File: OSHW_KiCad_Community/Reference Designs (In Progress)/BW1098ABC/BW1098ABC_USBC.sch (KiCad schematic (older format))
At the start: 36 parts, among them J10 USB3.1 TYPEC XKB-U262, J12 PJ-050AH or NEB21R, J13 DF23C-50DP-0.5V_92_, U6 USB Type-C Switch, U7 USB Type-C Port Control

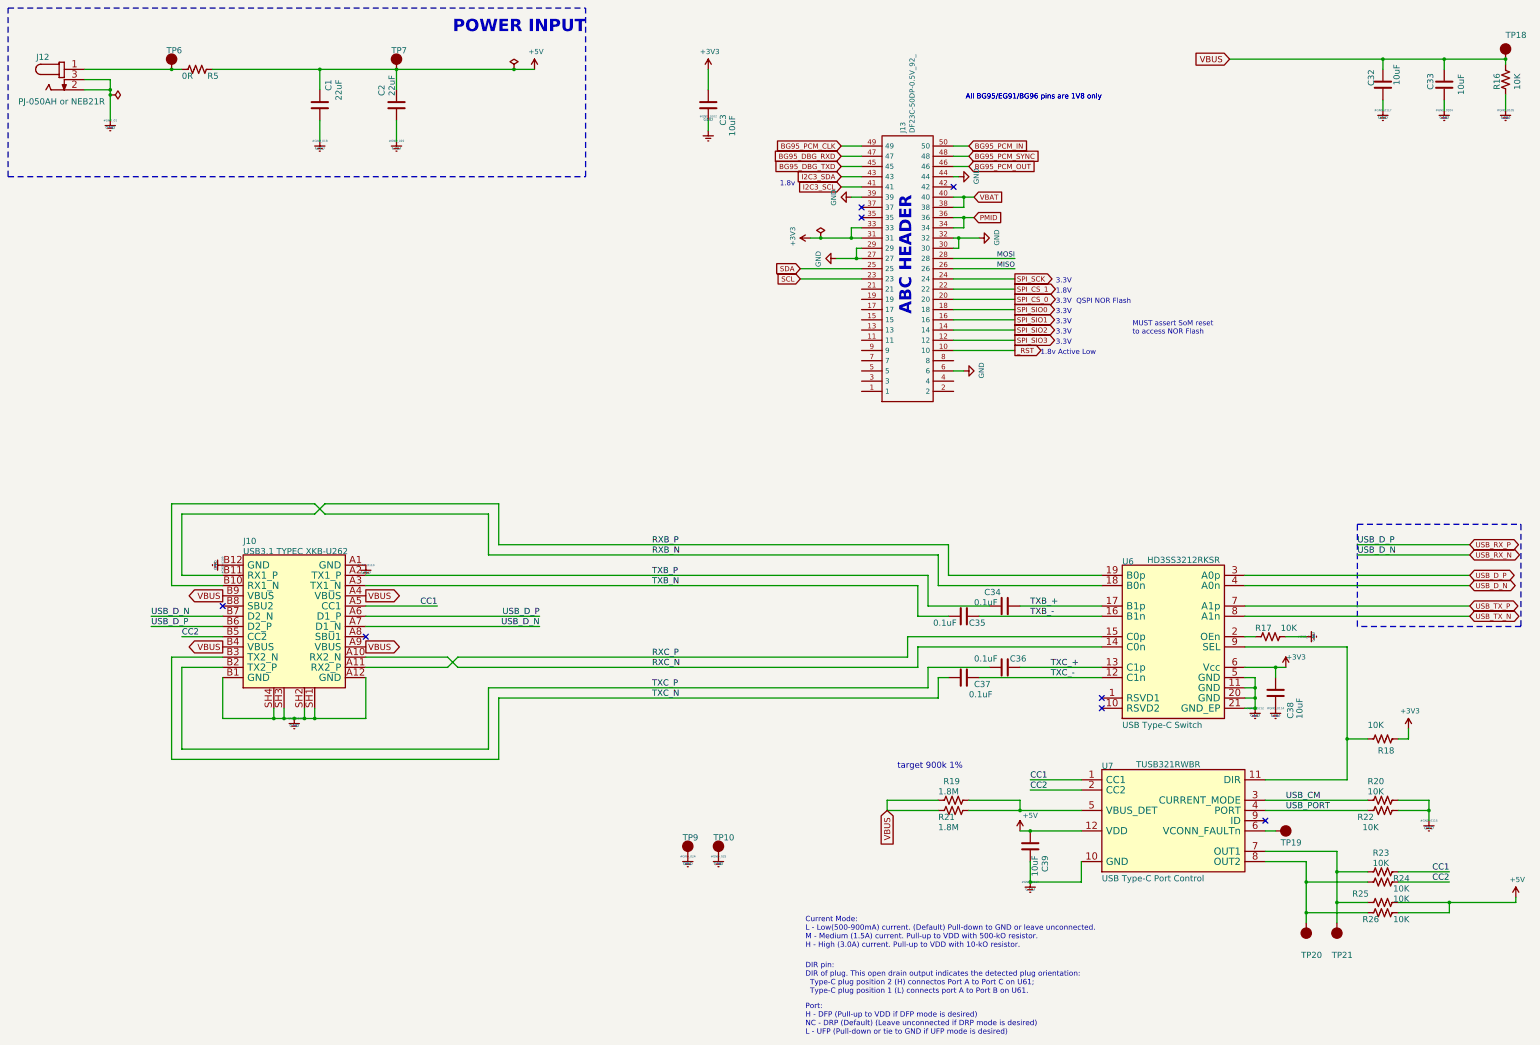
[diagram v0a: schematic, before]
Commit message: ABC Updates
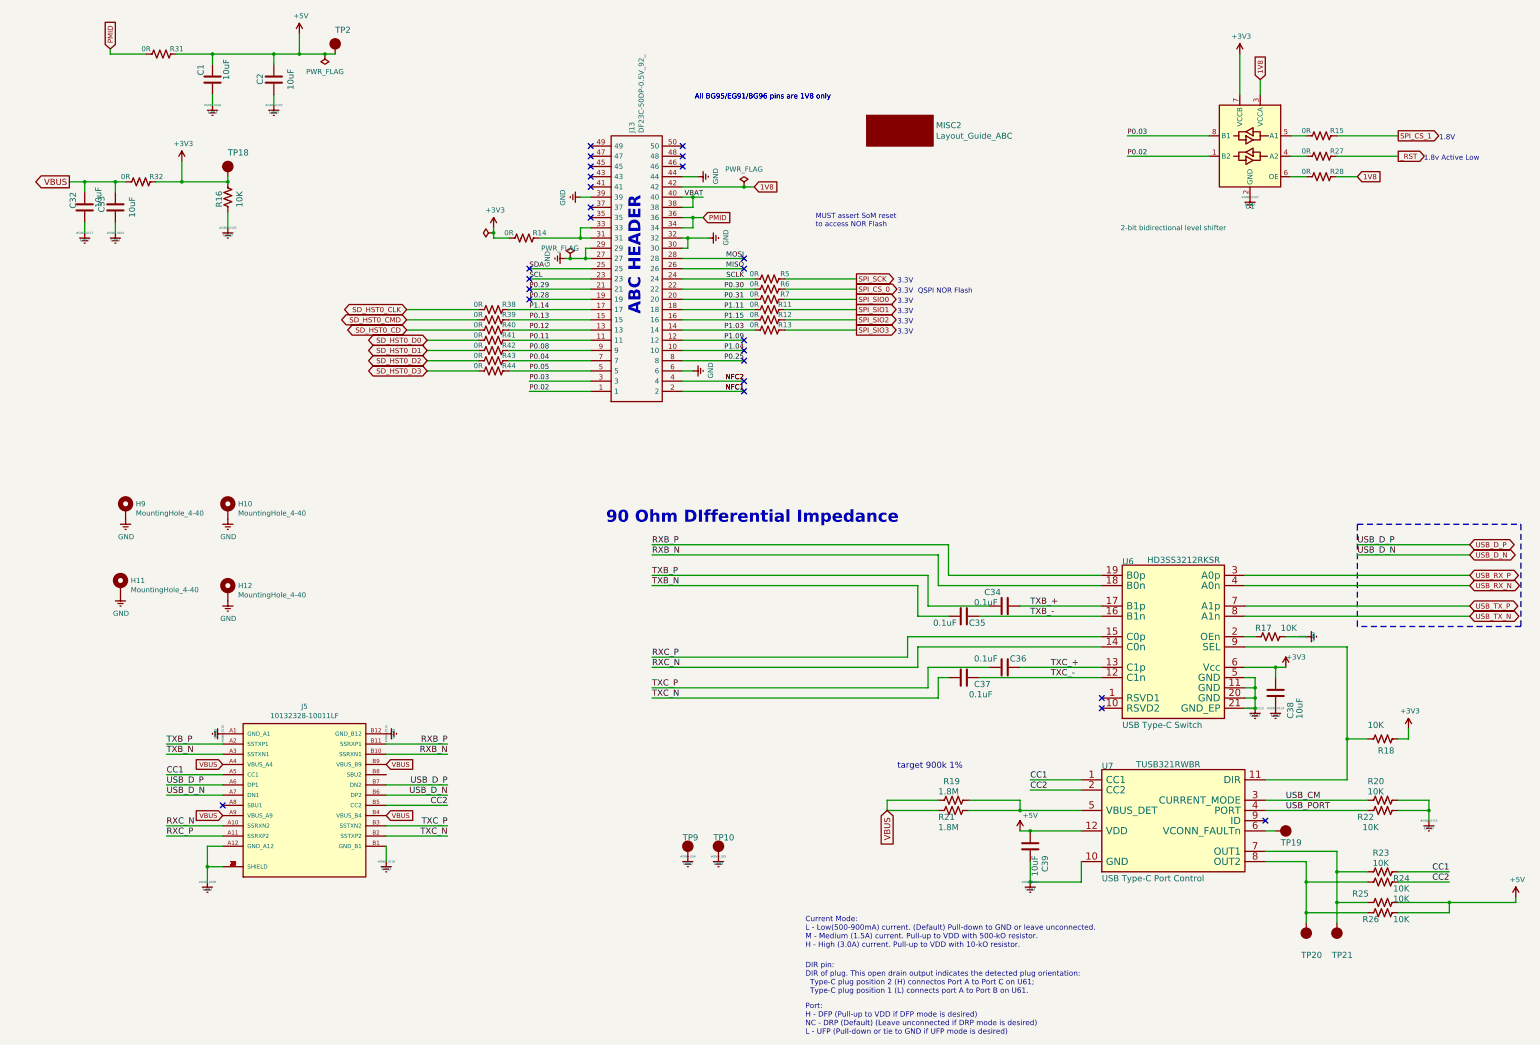
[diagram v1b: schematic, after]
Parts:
- removed C3: 10uF, Capacitor_SMD:C_0603_1608Metric, symbol Device:C
- removed J10: USB3.1 TYPEC XKB-U262, Connector_USB:USB_C_Receptacle_XKB_U262-16XN-4BVC11, symbol BW1098ABC-rescue:105450-0101-DEPTH
- removed J12: PJ-050AH or NEB21R, Connector_BarrelJack:BarrelJack_CUI_PJ-063AH_Horizontal, symbol BW1098ABC-rescue:PJ-050AH_NEB21R_COMBO-depthAI_sch
- removed TP6, TP7: TEST_POINT, TestPoint:TestPoint_Pad_1.0x1.0mm, symbol BW1098ABC-rescue:TEST_POINT-depthAI_sch
- added H10, H11, H12, H9: MountingHole_4-40, ABC:4881, symbol BW1098ABC-rescue:Mechanical_MountingHole_Pad-depthAI_sch
- added J5: 10132328-10011LF, AMPHENOL_10132328-10011LF, symbol 10132328-10011LF:10132328-10011LF
- added MISC2: Layout_Guide_ABC, ABC:ABC-Layout, symbol BW1098ABC-rescue:Layout_Guide_BW1099-DEPTH
- added R11, R12, R13, R14, R15, R27, R28, R31, R32, R38, R39, R40, R41, R42, R43, R44, R6, R7: 0R, Resistor_SMD:R_0603_1608Metric, symbol Device:R_US
- added TP2: ~, TestPoint:TestPoint_Pad_1.0x1.0mm, symbol BW1098ABC-rescue:TEST_POINT-DEPTH
- added U1: 2-bit bidirectional level shifter, Package_TO_SOT_SMD:SOT-23-8, symbol Logic_LevelTranslator:TXB0102DCT
- C1, C2: value 22uF -> 10uF; Voltage Rating 10V -> 6.3V
- U6: footprint Luxonis_KiCad_Master:Texas_Instruments-RKS0020A-0-0-MFG -> Luxonis_KiCad_Master:Texas_Instruments-HD3SS3212RKSR
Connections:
- net GND is gone; now on net Earth: J13.27, J13.29, J13.30, J13.32, J13.39, J13.44, J13.6
- net +3V3: now also R16.2, TP18.1 (P), R14.2, R32.1, U1.7 (VCCB); no longer J13.31, J13.33
- net +5V: now also R31.1, TP2.1 (P); no longer R5.1
- net CC1: now also J5.A5 (CC1)
- net CC2: now also J5.B5 (CC2)
- net Earth: now also H10.1, H11.1, H12.1, H9.1, J5.1 (SHIELD), J5.10 (SHIELD), J5.11 (SHIELD), J5.12 (SHIELD), J5.13 (SHIELD), J5.14 (SHIELD), J5.2 (SHIELD), J5.3 (SHIELD), J5.4 (SHIELD), J5.5 (SHIELD), J5.6 (SHIELD), J5.7 (SHIELD), J5.8 (SHIELD), J5.9 (SHIELD), J5.A1 (GND_A1), J5.A12 (GND_A12), J5.B1 (GND_B1), J5.B12 (GND_B12), U1.2 (GND)
- net PMID: now also R31.2
- net RXB_N: now also J5.B10 (SSRXN1)
- net RXB_P: now also J5.B11 (SSRXP1)
- net RXC_N: now also J5.A10 (SSRXN2)
- net RXC_P: now also J5.A11 (SSRXP2)
- net SPI_CS_0: now also R6.1; no longer J13.20
- net SPI_CS_1: now also R15.1; no longer J13.22
- net SPI_SCK: now also R5.1; no longer J13.24
- net SPI_SIO0: now also R7.1; no longer J13.18
- net SPI_SIO1: now also R11.1; no longer J13.16
- net SPI_SIO2: now also R12.1; no longer J13.14
- net SPI_SIO3: now also R13.1; no longer J13.12
- net TXB_N: now also J5.A3 (SSTXN1)
- net TXB_P: now also J5.A2 (SSTXP1)
- net TXC_N: now also J5.B2 (SSTXP2)
- net TXC_P: now also J5.B3 (SSTXN2)
- net USB_D_N: now also J5.A7 (DN1), J5.B6 (DP2); no longer U6.4 (A0n)
- net USB_D_P: now also J5.A6 (DP1), J5.B7 (DN2); no longer U6.3 (A0p)
- net VBUS: now also J5.A4 (VBUS_A4), J5.A9 (VBUS_A9), J5.B4 (VBUS_B4), J5.B9 (VBUS_B9), R32.2; no longer R16.2, TP18.1 (P)
- net _RST: now also R27.1; no longer J13.10
- net P0.02: now reaches J13.1
- net P0.02: now also U1.1 (B2)
- net P0.11: now reaches J13.11
- net P0.11: now also R41.1
- net P0.12: now reaches J13.13
- net P0.12: now also R40.1
- net P0.13: now reaches J13.15
- net P0.13: now also R39.1
- net P1.14: now reaches J13.17
- net P1.14: now also R38.1
- net P0.28: now reaches J13.19
- net NFC1: now reaches J13.2
- net P0.29: now reaches J13.21
- net P0.03: now reaches J13.3
- net P0.03: now also U1.8 (B1)
- net NFC2: now reaches J13.4
- net 1V8: now reaches J13.42
- net 1V8: now also R28.1, U1.3 (VCCA)
- net P0.05: now reaches J13.5
- net P0.05: now also R44.1
- net P0.04: now reaches J13.7
- net P0.04: now also R43.1
- net P0.25: now reaches J13.8
- net P0.08: now reaches J13.9
- net P0.08: now also R42.1
- net SCLK: now reaches R5.2
- net SCLK: now also J13.24
- net BG95_DBG_RXD: no longer names the net of J13.47
- net BG95_DBG_TXD: no longer names the net of J13.45
- net BG95_PCM_CLK: no longer names the net of J13.49
- net BG95_PCM_IN: no longer names the net of J13.50
- net BG95_PCM_OUT: no longer names the net of J13.46
- net BG95_PCM_SYNC: no longer names the net of J13.48
- net I2C3_SCL: no longer names the net of J13.41
- net I2C3_SDA: no longer names the net of J13.43
- new net: R27.2, U1.4 (A2)
- new net: R15.2, U1.5 (A1)
- new net: R28.2, U1.6 (OE)
- new net: J13.31, J13.33, R14.1
- new net P0.30: J13.22, R6.2
- new net P0.31: J13.20, R7.2
- new net P1.03: J13.14, R13.2
- new net P1.04: J13.10
- new net P1.09: J13.12
- new net P1.11: J13.18, R11.2
- new net P1.15: J13.16, R12.2
- new net SD_HST0_CD: R40.2
- new net SD_HST0_CLK: R38.2
- new net SD_HST0_CMD: R39.2
- new net SD_HST0_D0: R41.2
- new net SD_HST0_D1: R42.2
- new net SD_HST0_D2: R43.2
- new net SD_HST0_D3: R44.2
- new net USB_RX_N: U6.4 (A0n)
- new net USB_RX_P: U6.3 (A0p)
- no-connect marks 8 -> 25
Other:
- note added: "90 Ohm DIfferential Impedance"
- note removed: "1.8v"
- note removed: "POWER INPUT"
- moved on the sheet: C32, C33, J13, R16, TP18
